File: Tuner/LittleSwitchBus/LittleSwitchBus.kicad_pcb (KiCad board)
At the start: 2 copper layers, 100 x 100 mm, 99 parts, among them J1 Conn_Coaxial, J10 Conn_Coaxial, J11 Conn_02x05_Odd_Even, J13 Conn_01x01, J14 Conn_01x01, J15 Conn_01x01, J16 Conn_01x01, J2 Conn_Coaxial, J3 Conn_Coaxial, J4 Conn_Coaxial, J5 Conn_Coaxial, J6 Conn_Coaxial, J7 Conn_Coaxial, J8 Conn_Coaxial, J9 Conn_Coaxial, U1 MCP23008, U2 ULN2803A

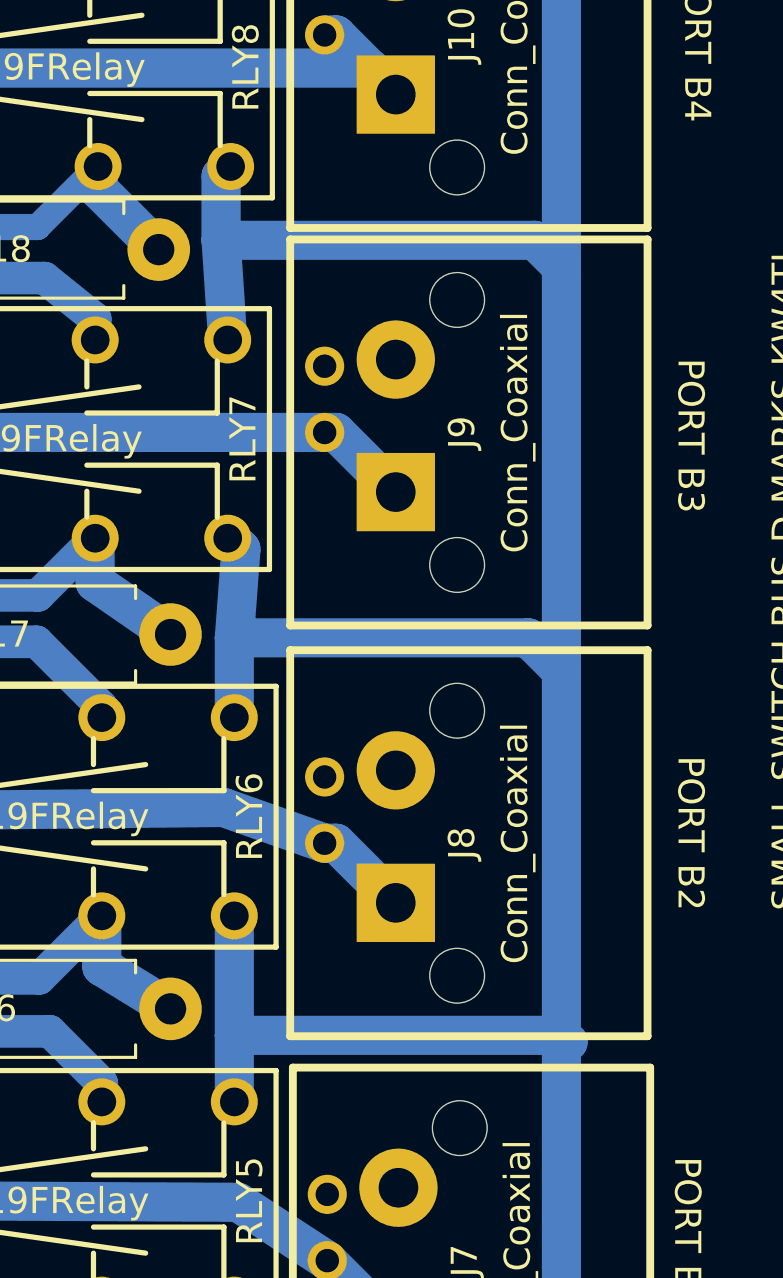
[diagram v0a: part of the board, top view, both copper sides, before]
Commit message: Added some fixes to tuner code
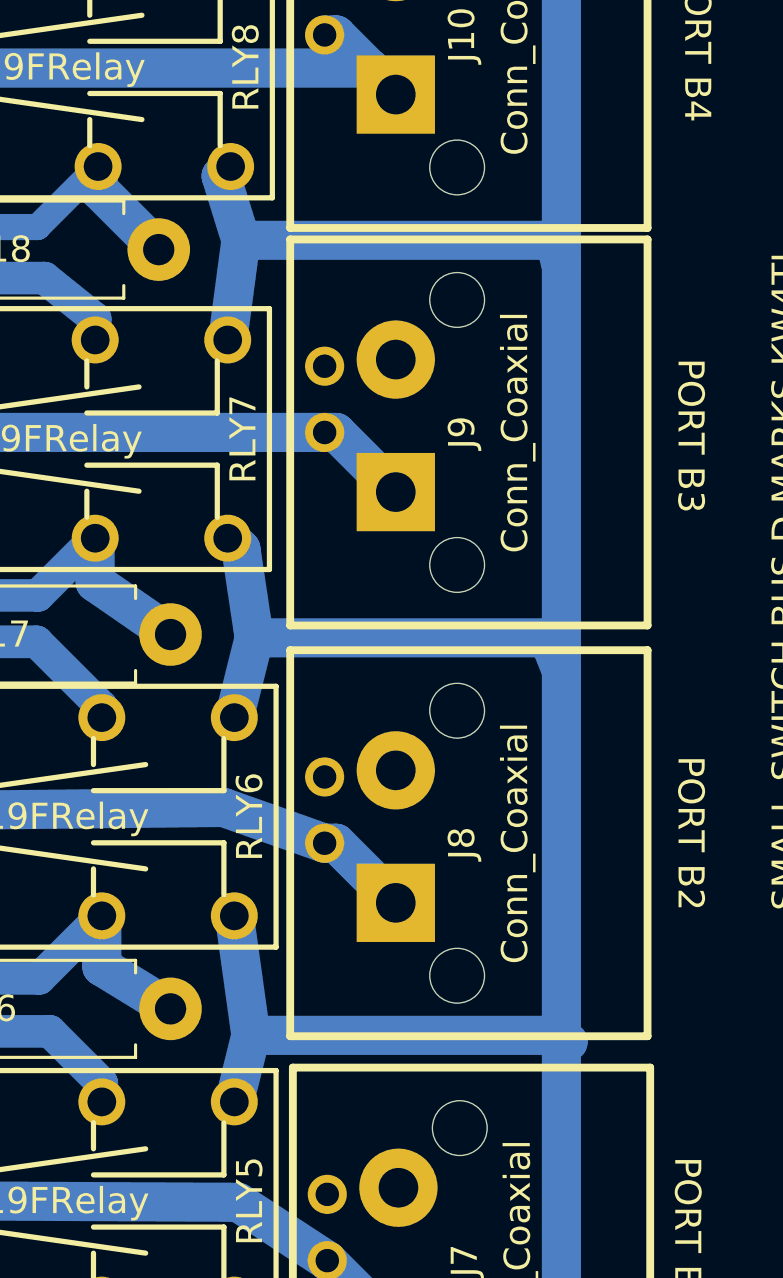
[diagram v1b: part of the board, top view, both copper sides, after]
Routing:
- net Net-(J6-Pad1): track 163.3 -> 162.3 mm
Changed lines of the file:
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@@
   (segment (start 120.904 54.356) (end 120.904 56.60884) (width 1.5) (layer B.Cu) (net 7) (status 10))
   (segment (start 120.904 56.60884) (end 124.47776 60.1826) (width 1.5) (layer B.Cu) (net 7))
-  (segment (start 124.112 70.612) (end 136.144 70.612) (width 1.5) (layer B.Cu) (net 7))
-  (segment (start 136.144 70.612) (end 137.16 71.628) (width 1.5) (layer B.Cu) (net 7))
-  (segment (start 124.366 74.432) (end 124.112 70.612) (width 1.5) (layer B.Cu) (net 7) (status 10))
-  (segment (start 124.112 70.612) (end 124.112 68.14836) (width 1.5) (layer B.Cu) (net 7))
+  (segment (start 124.874 70.612) (end 136.906 70.612) (width 1.5) (layer B.Cu) (net 7))
+  (segment (start 136.906 70.612) (end 137.16 71.628) (width 1.5) (layer B.Cu) (net 7))
+  (segment (start 124.366 74.432) (end 124.874 70.612) (width 1.5) (layer B.Cu) (net 7) (status 10))
+  (segment (start 124.874 70.612) (end 124.112 68.14836) (width 1.5) (layer B.Cu) (net 7))
   (segment (start 124.112 68.14836) (end 124.47776 67.7826) (width 1.5) (layer B.Cu) (net 7))
-  (segment (start 124.62 85.852) (end 135.89 85.852) (width 1.5) (layer B.Cu) (net 7))
-  (segment (start 135.89 85.852) (end 137.16 87.122) (width 1.5) (layer B.Cu) (net 7))
-  (segment (start 124.62 88.91) (end 124.62 85.852) (width 1.5) (layer B.Cu) (net 7))
-  (segment (start 124.62 85.852) (end 124.874 82.456) (width 1.5) (layer B.Cu) (net 7) (status 20))
+  (segment (start 125.382 85.852) (end 136.652 85.852) (width 1.5) (layer B.Cu) (net 7))
+  (segment (start 136.652 85.852) (end 137.16 87.122) (width 1.5) (layer B.Cu) (net 7))
+  (segment (start 124.62 88.91) (end 125.382 85.852) (width 1.5) (layer B.Cu) (net 7))
+  (segment (start 125.382 85.852) (end 124.874 82.456) (width 1.5) (layer B.Cu) (net 7) (status 20))
   (segment (start 124.874 82.456) (end 124.45 82.032) (width 1.5) (layer B.Cu) (net 7) (status 30))
   (segment (start 124.45 82.032) (end 124.366 82.032) (width 1.5) (layer B.Cu) (net 7) (status 30))
-  (segment (start 124.62 101.092) (end 136.906 101.092) (width 1.5) (layer B.Cu) (net 7))
+  (segment (start 125.255 101.092) (end 136.906 101.092) (width 1.5) (layer B.Cu) (net 7))
   (segment (start 136.906 101.092) (end 137.16 101.346) (width 1.5) (layer B.Cu) (net 7))
-  (segment (start 124.62 103.642) (end 124.62 101.092) (width 1.5) (layer B.Cu) (net 7))
-  (segment (start 124.62 101.092) (end 124.62 96.51) (width 1.5) (layer B.Cu) (net 7))
+  (segment (start 124.62 103.642) (end 125.255 101.092) (width 1.5) (layer B.Cu) (net 7))
+  (segment (start 125.255 101.092) (end 124.62 96.51) (width 1.5) (layer B.Cu) (net 7))
   (segment (start 137.16 101.346) (end 137.414 101.346) (width 1.5) (layer B.Cu) (net 7))
   (segment (start 137.414 101.346) (end 137.16 101.346) (width 1.5) (layer B.Cu) (net 7))
